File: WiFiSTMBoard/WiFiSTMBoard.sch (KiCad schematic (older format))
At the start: 22 parts

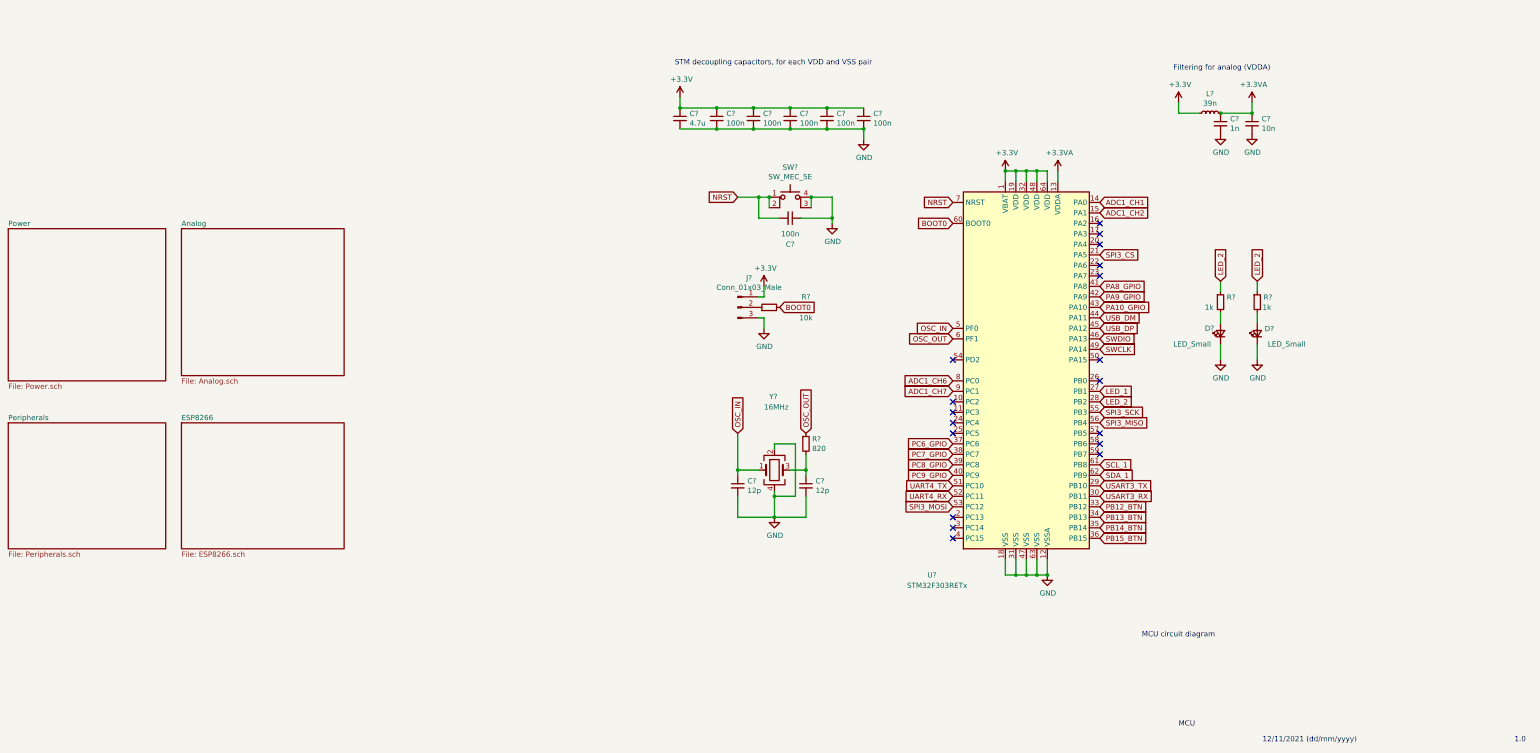
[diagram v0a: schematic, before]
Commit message: added input
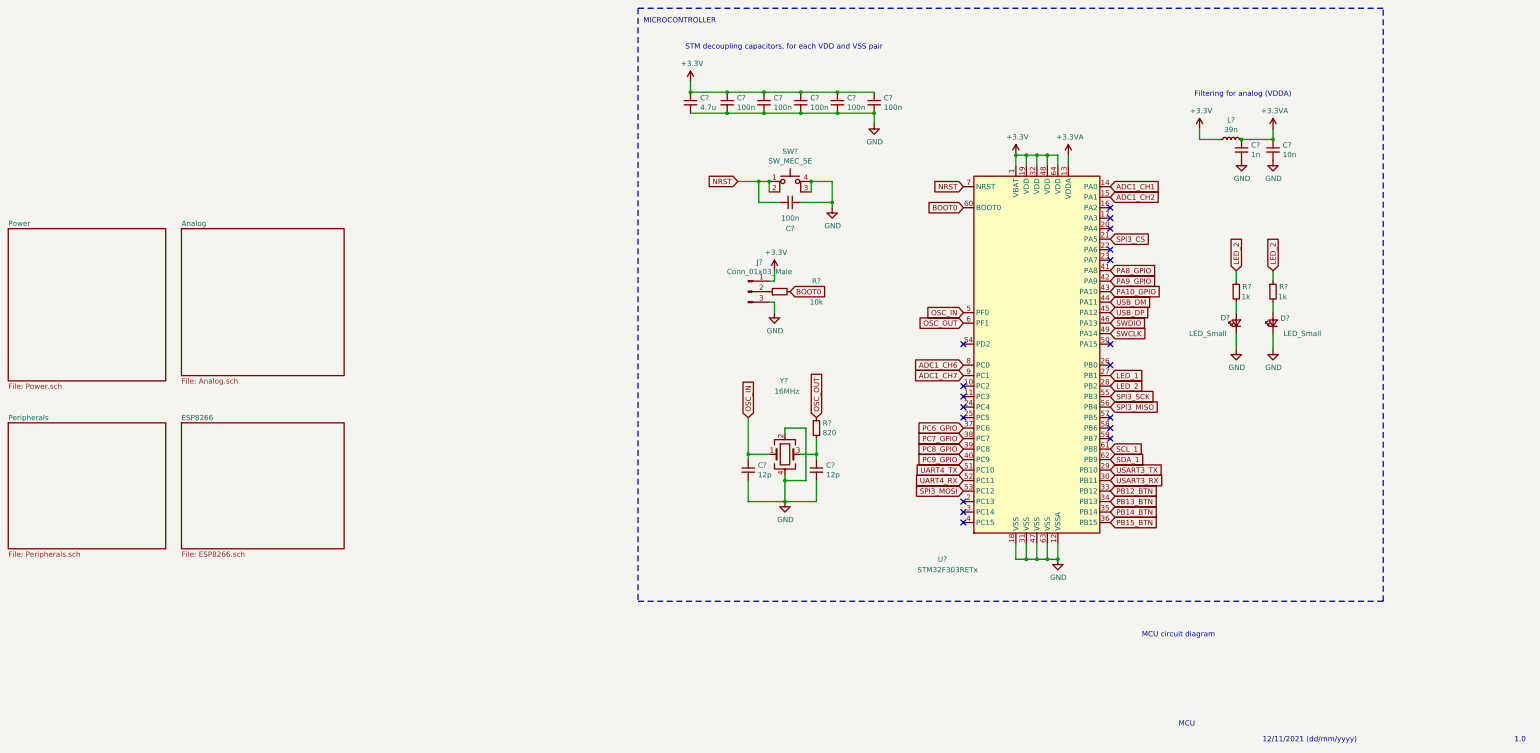
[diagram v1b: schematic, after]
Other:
- note added: "MICROCONTROLLER"
- moved on the sheet: C?, D?, J?, L?, R?, SW?, U?, Y?
